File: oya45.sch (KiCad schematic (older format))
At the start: 106 parts, among them U1 ProMicro

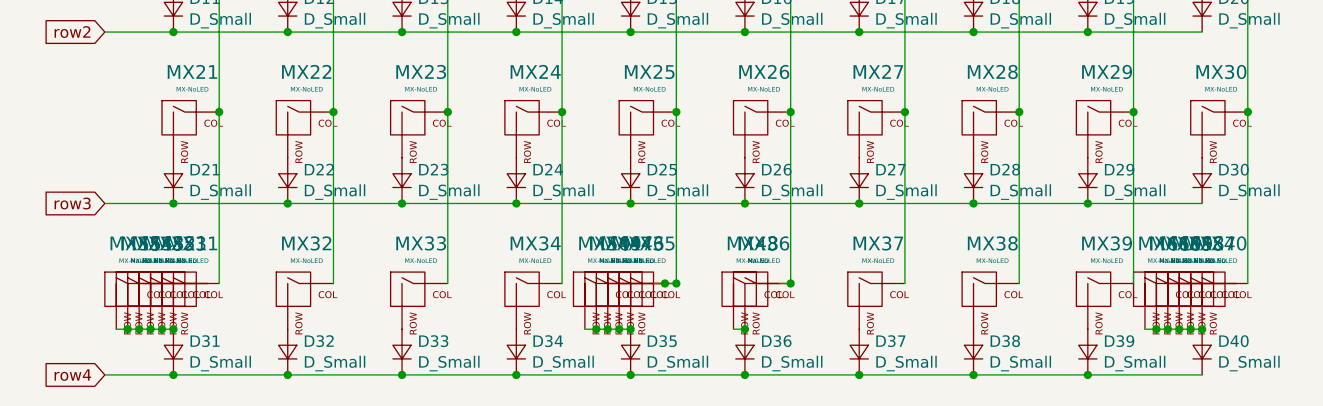
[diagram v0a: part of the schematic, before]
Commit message: finished pcb
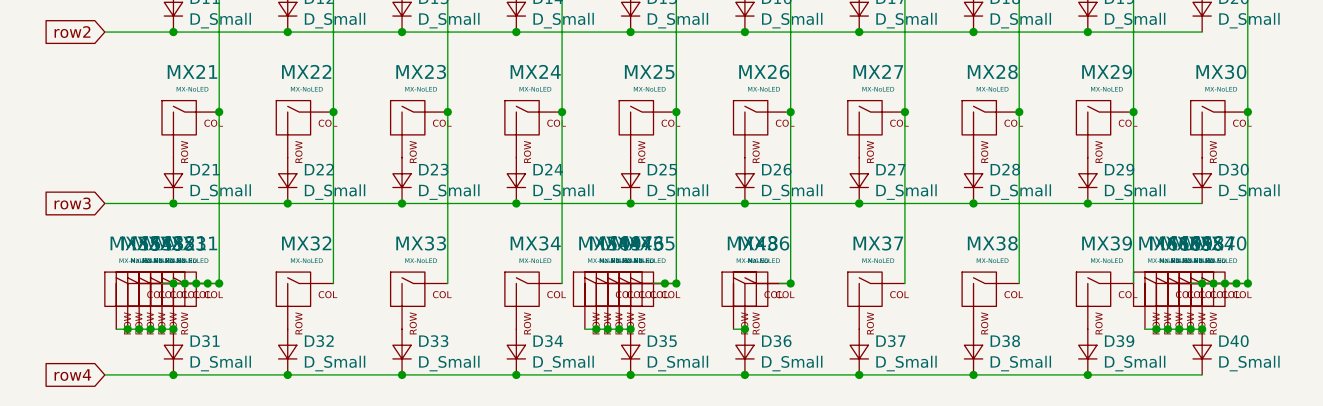
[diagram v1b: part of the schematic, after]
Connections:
- net col0: now also MX51.1 (COL), MX52.1 (COL), MX53.1 (COL), MX54.1 (COL), MX55.1 (COL)
- net col9: now also MX57.1 (COL), MX58.1 (COL), MX59.1 (COL), MX60.1 (COL), MX61.1 (COL)
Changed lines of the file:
@@
 Wire Wire Line
 	10000 5000 9950 5000
+Wire Wire Line
+	10250 4800 10200 4800
+Connection ~ 10250 4800
+Connection ~ 10050 4800
+Wire Wire Line
+	10050 4800 10000 4800
+Connection ~ 10100 4800
+Wire Wire Line
+	10100 4800 10050 4800
+Connection ~ 10150 4800
+Wire Wire Line
+	10150 4800 10100 4800
+Connection ~ 10200 4800
+Wire Wire Line
+	10200 4800 10150 4800
+Wire Wire Line
+	5750 4800 5700 4800
+Connection ~ 5750 4800
+Connection ~ 5550 4800
+Wire Wire Line
+	5550 4800 5500 4800
+Connection ~ 5600 4800
+Wire Wire Line
+	5600 4800 5550 4800
+Connection ~ 5650 4800
+Wire Wire Line
+	5650 4800 5600 4800
+Connection ~ 5700 4800
+Wire Wire Line
+	5700 4800 5650 4800
 $EndSCHEMATC
